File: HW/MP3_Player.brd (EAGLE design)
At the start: 160 x 20 mm, 76 parts, among them J1 ISP/SPI, J2 LIPO-BATTERY-CONNECTOR, J3 USD-SDIO-SOCKETJLH, Q2 12.288MHz, U1 3.3V/150mA, U2 1.8V/100mA, U3 ATMEGA32U2, U4 VS1053B, U5 MCP73831, X2 USBSMD

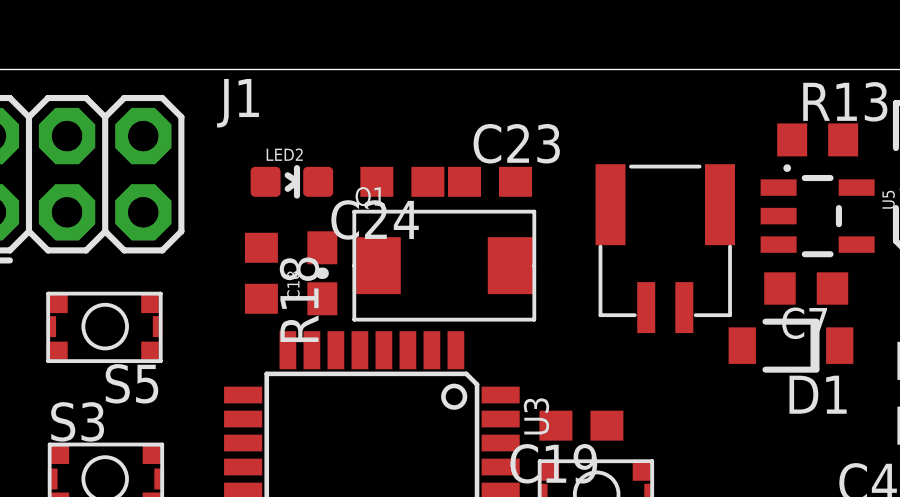
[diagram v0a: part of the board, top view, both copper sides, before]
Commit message: Comit before 1st autorouter
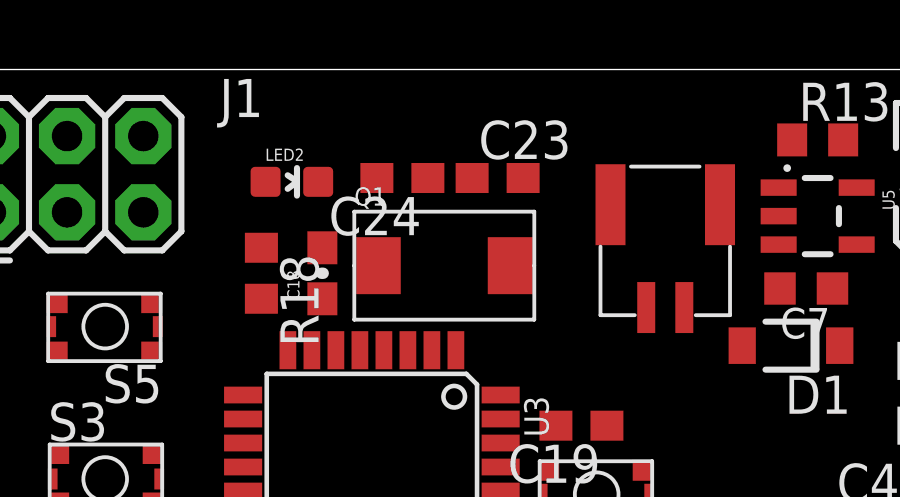
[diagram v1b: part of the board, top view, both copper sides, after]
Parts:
- moved C23 0.28 mm to (132.5, 16.4)
- moved C24 0.13 mm to (129.3, 16.4)
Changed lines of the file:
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@@
 </class>
 </classes>
-<designrules name="default">
+<designrules name="default *">
 <description language="de">&lt;b&gt;EAGLE Design Rules&lt;/b&gt;
 &lt;p&gt;
@@
 <param name="mtCopper" value="0.035mm 0.035mm 0.035mm 0.035mm 0.035mm 0.035mm 0.035mm 0.035mm 0.035mm 0.035mm 0.035mm 0.035mm 0.035mm 0.035mm 0.035mm 0.035mm"/>
 <param name="mtIsolate" value="1.5mm 0.15mm 0.2mm 0.15mm 0.2mm 0.15mm 0.2mm 0.15mm 0.2mm 0.15mm 0.2mm 0.15mm 0.2mm 0.15mm 0.2mm"/>
-<param name="mdWireWire" value="8mil"/>
-<param name="mdWirePad" value="8mil"/>
-<param name="mdWireVia" value="8mil"/>
-<param name="mdPadPad" value="8mil"/>
-<param name="mdPadVia" value="8mil"/>
-<param name="mdViaVia" value="8mil"/>
+<param name="mdWireWire" value="10mil"/>
+<param name="mdWirePad" value="10mil"/>
+<param name="mdWireVia" value="10mil"/>
+<param name="mdPadPad" value="2mil"/>
+<param name="mdPadVia" value="10mil"/>
+<param name="mdViaVia" value="10mil"/>
 <param name="mdSmdPad" value="8mil"/>
 <param name="mdSmdVia" value="8mil"/>
-<param name="mdSmdSmd" value="8mil"/>
+<param name="mdSmdSmd" value="2mil"/>
 <param name="mdViaViaSameLayer" value="8mil"/>
 <param name="mnLayersViaInSmd" value="2"/>
-<param name="mdCopperDimension" value="40mil"/>
-<param name="mdDrill" value="8mil"/>
+<param name="mdCopperDimension" value="0mil"/>
+<param name="mdDrill" value="10mil"/>
 <param name="mdSmdStop" value="0mil"/>
 <param name="msWidth" value="10mil"/>
@@
 <element name="U3" library="hf" package="TQFP32-08" value="ATMEGA32U2" x="128.27" y="6.35" rot="R270"/>
 <element name="C22" library="rcl" package="C0603" value="1u" x="135.255" y="3.429"/>
-<element name="C23" library="rcl" package="C0603" value="18p" x="132.207" y="16.256"/>
-<element name="C24" library="rcl" package="C0603" value="18p" x="129.286" y="16.256" rot="R180"/>
+<element name="C23" library="rcl" package="C0603" value="18p" x="132.461" y="16.383"/>
+<element name="C24" library="rcl" package="C0603" value="18p" x="129.286" y="16.383" rot="R180"/>
 <element name="R23" library="rcl" package="R0603" value="22" x="148.082" y="9.398" rot="R180"/>
 <element name="R24" library="rcl" package="R0603" value="22" x="148.082" y="11.557" rot="R180"/>
@@
 <wire x1="137.414" y1="12.065" x2="141.8289" y2="15.113" width="0" layer="19" extent="1-16"/>
 <wire x1="141.873" y1="12.7" x2="141.8289" y2="15.113" width="0" layer="19" extent="1-1"/>
-<wire x1="131.357" y1="16.256" x2="137.414" y2="12.065" width="0" layer="19" extent="1-16"/>
-<wire x1="130.136" y1="16.256" x2="131.357" y2="16.256" width="0" layer="19" extent="1-1"/>
-<wire x1="126.48" y1="16.256" x2="130.136" y2="16.256" width="0" layer="19" extent="1-1"/>
+<wire x1="131.611" y1="16.383" x2="137.414" y2="12.065" width="0" layer="19" extent="1-16"/>
+<wire x1="130.136" y1="16.383" x2="131.611" y2="16.383" width="0" layer="19" extent="1-1"/>
+<wire x1="126.48" y1="16.256" x2="130.136" y2="16.383" width="0" layer="19" extent="1-1"/>
 <wire x1="126.619" y1="14.058" x2="126.48" y2="16.256" width="0" layer="19" extent="1-1"/>
 <wire x1="129.47" y1="10.6426" x2="126.619" y2="14.058" width="0" layer="19" extent="1-1"/>
@@
 <contactref element="C23" pad="2"/>
 <contactref element="Q1" pad="P$2"/>
-<wire x1="131.07" y1="10.6426" x2="133.057" y2="16.256" width="0" layer="19" extent="1-1"/>
+<wire x1="131.07" y1="10.6426" x2="133.311" y2="16.383" width="0" layer="19" extent="1-1"/>
 <wire x1="132.883" y1="13.462" x2="131.07" y2="10.6426" width="0" layer="19" extent="1-1"/>
 </signal>
@@
 <contactref element="C24" pad="2"/>
 <contactref element="Q1" pad="P$1"/>
-<wire x1="130.27" y1="10.6426" x2="128.436" y2="16.256" width="0" layer="19" extent="1-1"/>
+<wire x1="130.27" y1="10.6426" x2="128.436" y2="16.383" width="0" layer="19" extent="1-1"/>
 <wire x1="128.483" y1="13.462" x2="130.27" y2="10.6426" width="0" layer="19" extent="1-1"/>
 </signal>
@@
 </signal>
 </signals>
+<errors>
+</errors>
 </board>
 </drawing>
